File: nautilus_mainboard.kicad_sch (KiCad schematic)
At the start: 10 parts

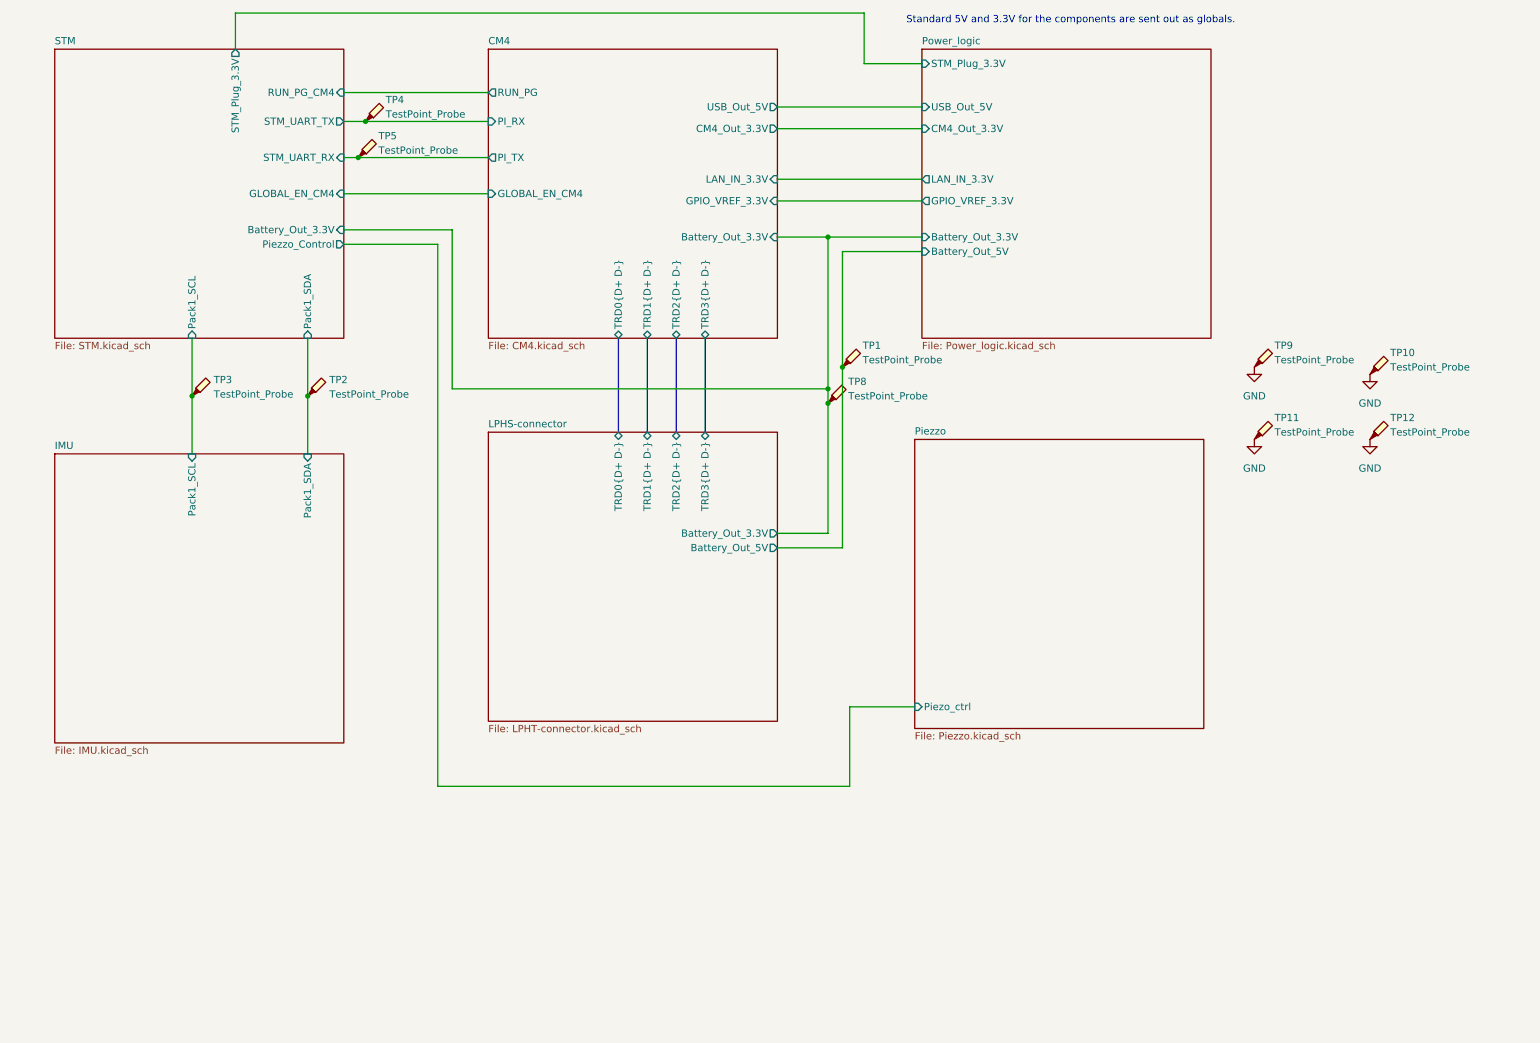
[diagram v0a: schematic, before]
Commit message: chore: Loads of redoing stuff. Added a Changelog
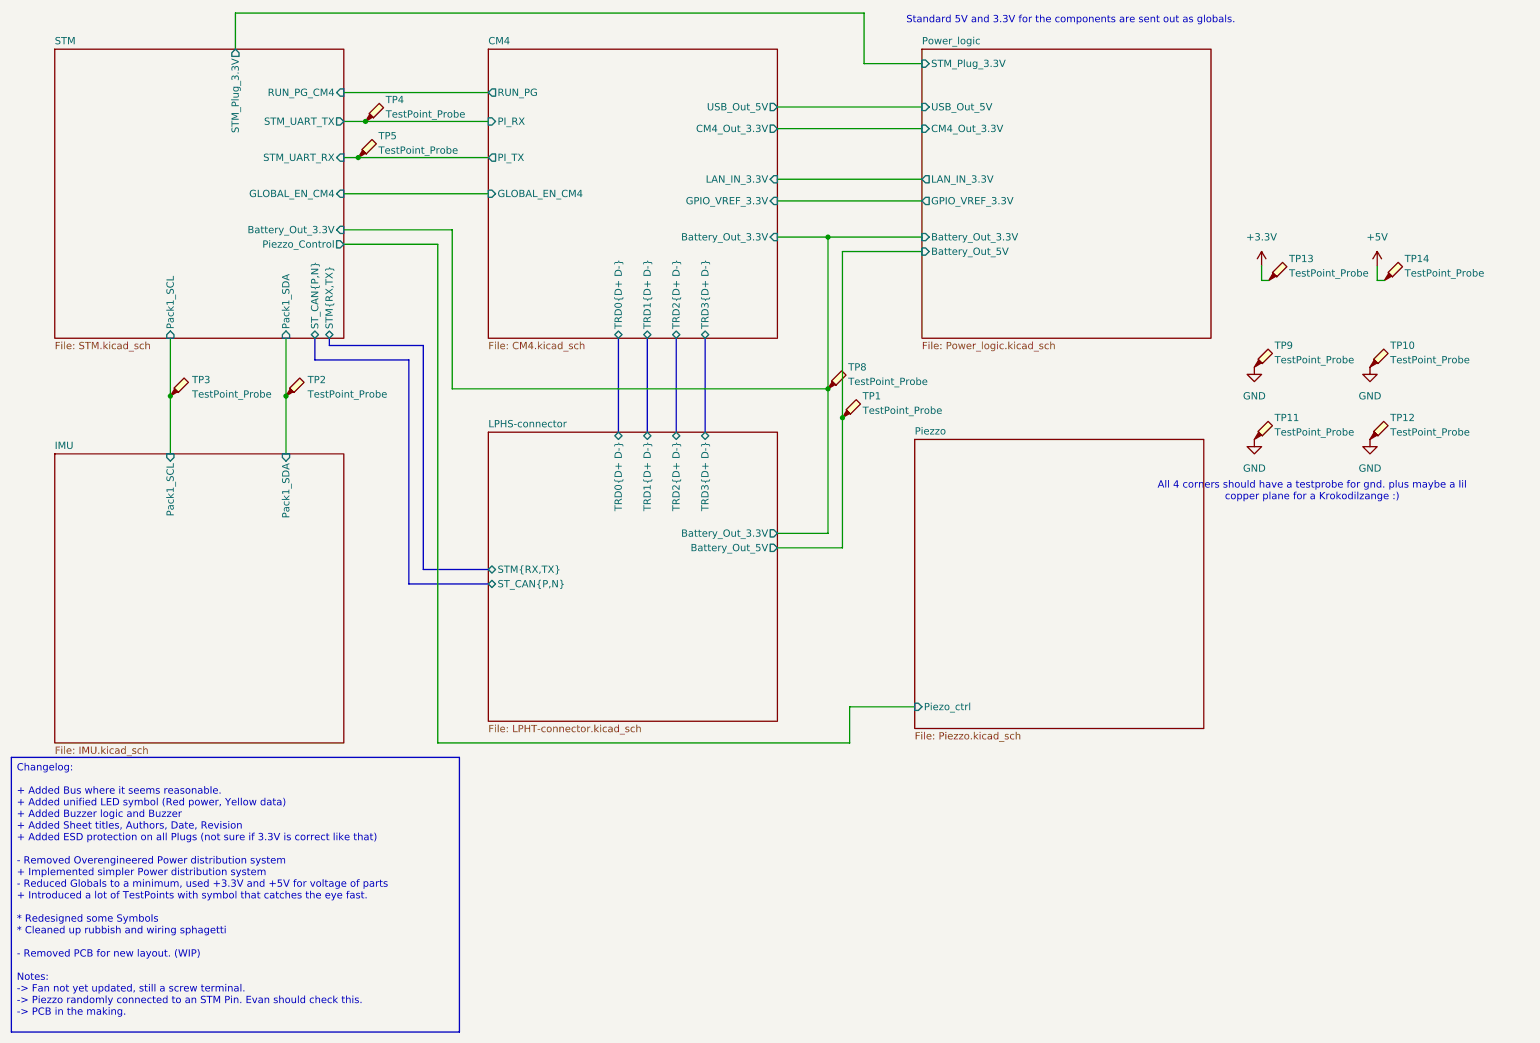
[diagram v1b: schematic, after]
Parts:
- added TP13, TP14: TestPoint_Probe, TestPoint:TestPoint_Pad_D1.0mm, symbol Connector:TestPoint_Probe
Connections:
- new net +3.3V: TP13.1
- new net +5V: TP14.1
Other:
- sheet LPHS-connector ports: added STM{RX,TX}, ST_CAN{P,N}; removed none
- sheet STM ports: added STM{RX,TX}, ST_CAN{P,N}; removed none
- note added: "All 4 corners should have a testprobe for gnd. plus maybe a lil copper plane for a Krokodilzange :)"
- title: (none) -> Nautilus_Mainboard
- moved on the sheet: TP1, TP10, TP2, TP3, TP8
